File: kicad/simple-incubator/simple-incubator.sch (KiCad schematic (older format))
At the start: 17 parts, among them J1 Conn_Coaxial_Power, J2 Fan, J3 Onewire1, J4 FT232L, J5 Onewire2, Q1 BSP75, Q2 IRF3704, SW1 Rotary_Encoder_Switch, U1 MCP1703A-5002_SOT223, U2 ATmega328-AU

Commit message: update kicad
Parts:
- Q1: symbol BSP75:BSP75 -> simple-incubator-rescue:BSP75-BSP75
- R2: footprint (none) -> Resistor_SMD:R_0805_2012Metric_Pad1.15x1.40mm_HandSolder
- SP1: symbol ICSP:ICSP -> simple-incubator-rescue:ICSP-ICSP
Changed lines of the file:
@@
 $EndComp
 $Comp
-L BSP75:BSP75 Q1
+L simple-incubator-rescue:BSP75-BSP75 Q1
 U 1 1 5C8944AE
 P 6950 2900
@@
 $EndComp
 $Comp
-L ICSP:ICSP SP1
+L simple-incubator-rescue:ICSP-ICSP SP1
 U 1 1 5C8952B3
 P 2550 5100
@@
 	9050 2950 9200 2950
 $Comp
-L power:GND #PWR?
+L power:GND #PWR0114
 U 1 1 5C89B676
 P 9200 2950
-F 0 "#PWR?" H 9200 2700 50  0001 C CNN
+F 0 "#PWR0114" H 9200 2700 50  0001 C CNN
 F 1 "GND" H 9205 2777 50  0000 C CNN
 F 2 "" H 9200 2950 50  0001 C CNN
@@
 F 0 "R2" V 9143 2850 50  0000 C CNN
 F 1 "R" V 9234 2850 50  0000 C CNN
-F 2 "" V 9280 2850 50  0001 C CNN
+F 2 "Resistor_SMD:R_0805_2012Metric_Pad1.15x1.40mm_HandSolder" V 9280 2850 50  0001 C CNN
 F 3 "~" H 9350 2850 50  0001 C CNN
 	1    9350 2850
@@
 	9250 2200 8650 2200
 $Comp
-L power:VCC #PWR?
+L power:VCC #PWR0115
 U 1 1 5C89FAE2
 P 8650 1850
-F 0 "#PWR?" H 8650 1700 50  0001 C CNN
+F 0 "#PWR0115" H 8650 1700 50  0001 C CNN
 F 1 "VCC" H 8667 2023 50  0000 C CNN
 F 2 "" H 8650 1850 50  0001 C CNN
@@
 RESET
 $Comp
-L power:GND #PWR?
+L power:GND #PWR0116
 U 1 1 5C8ACF03
 P 3200 5250
-F 0 "#PWR?" H 3200 5000 50  0001 C CNN
+F 0 "#PWR0116" H 3200 5000 50  0001 C CNN
 F 1 "GND" H 3205 5077 50  0000 C CNN
 F 2 "" H 3200 5250 50  0001 C CNN
@@
 	3350 3550 3550 3550
 $Comp
-L power:GND #PWR?
+L power:GND #PWR0117
 U 1 1 5C8B7EBD
 P 3550 3350
-F 0 "#PWR?" H 3550 3100 50  0001 C CNN
+F 0 "#PWR0117" H 3550 3100 50  0001 C CNN
 F 1 "GND" H 3555 3177 50  0000 C CNN
 F 2 "" H 3550 3350 50  0001 C CNN
@@
 	2750 3450 2200 3450
 $Comp
-L power:GND #PWR?
+L power:GND #PWR0118
 U 1 1 5C8BA7E6
 P 2200 3450
-F 0 "#PWR?" H 2200 3200 50  0001 C CNN
+F 0 "#PWR0118" H 2200 3200 50  0001 C CNN
 F 1 "GND" H 2205 3277 50  0000 C CNN
 F 2 "" H 2200 3450 50  0001 C CNN

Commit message: The footprint should have changed to simple footprint design with 9 pads and a hole.
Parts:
- Q1: symbol simple-incubator-rescue:BSP75-BSP75 -> simple-incubator-rescue:BSP75-BSP75-simple-incubator-rescue
- SP1: symbol simple-incubator-rescue:ICSP-ICSP -> simple-incubator-rescue:ICSP-ICSP-simple-incubator-rescue
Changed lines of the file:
@@
 $EndComp
 $Comp
-L simple-incubator-rescue:BSP75-BSP75 Q1
+L simple-incubator-rescue:BSP75-BSP75-simple-incubator-rescue Q1
 U 1 1 5C8944AE
 P 6950 2900
@@
 $EndComp
 $Comp
-L simple-incubator-rescue:ICSP-ICSP SP1
+L simple-incubator-rescue:ICSP-ICSP-simple-incubator-rescue SP1
 U 1 1 5C8952B3
 P 2550 5100

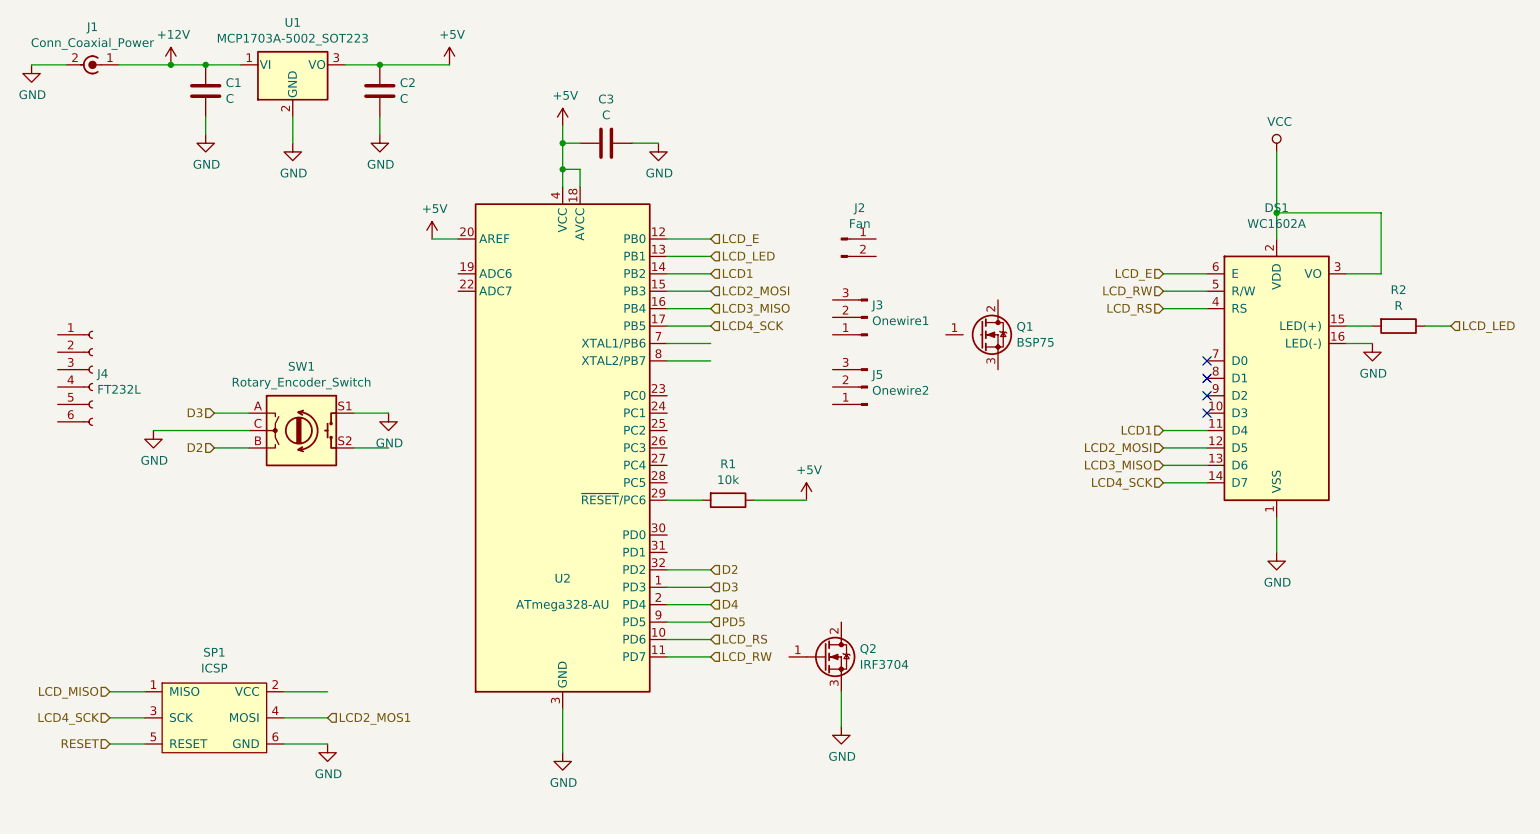
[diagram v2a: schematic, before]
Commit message: last weeks updates
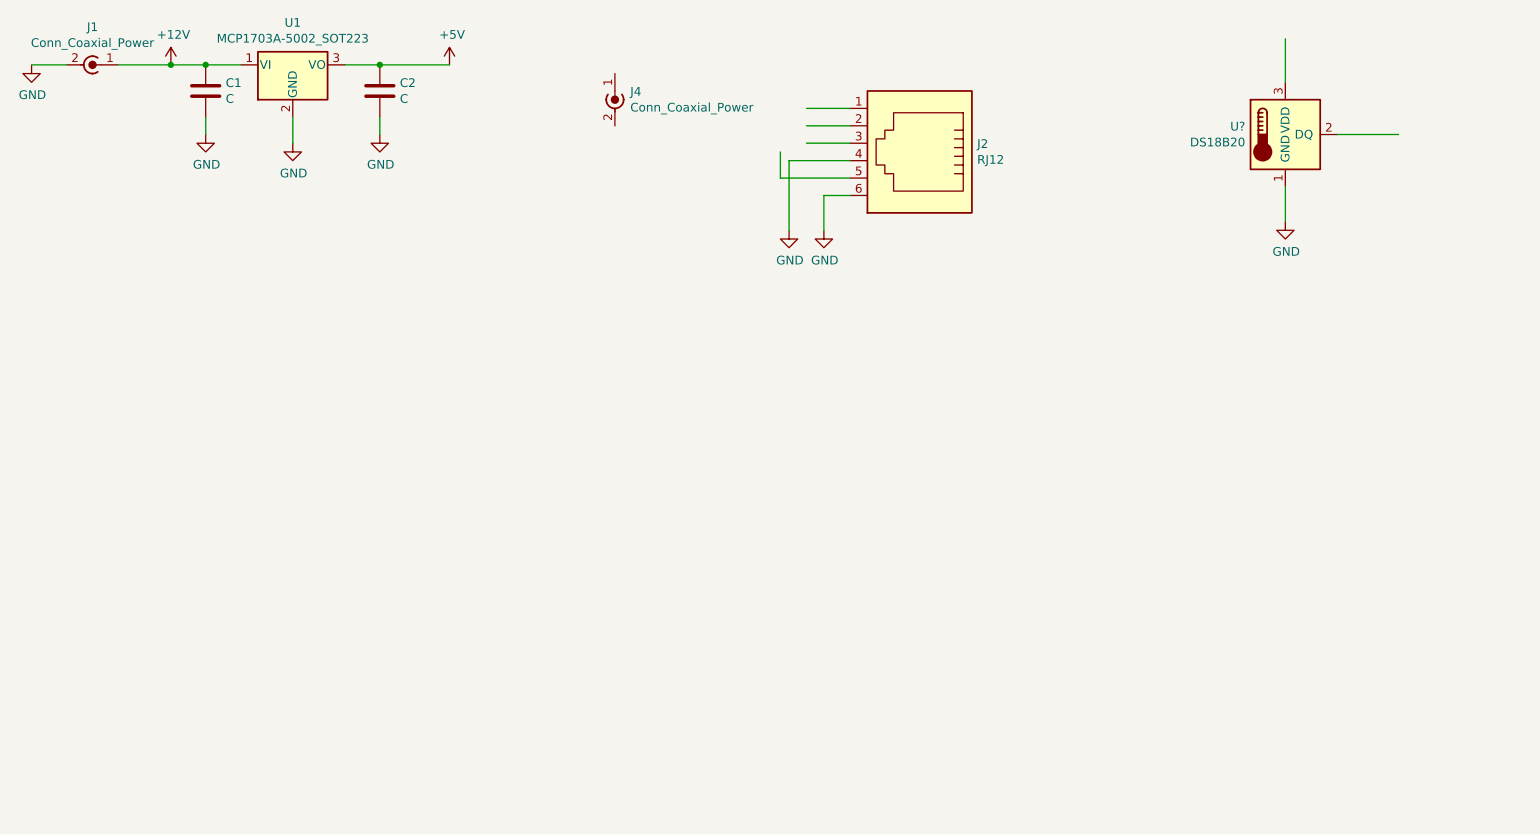
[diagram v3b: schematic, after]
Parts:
- removed C3: C, Capacitor_SMD:C_0805_2012Metric_Pad1.15x1.40mm_HandSolder, symbol Device:C
- removed DS1: WC1602A, Display:WC1602A, symbol Display_Character:WC1602A
- removed J2: Fan, Connector_BarrelJack:BarrelJack_Horizontal, symbol Connector:Conn_01x02_Male
- removed J3: Onewire1, Connector_Molex:Molex_KK-254_AE-6410-03A_1x03_P2.54mm_Vertical, symbol Connector:Conn_01x03_Male
- removed J4: FT232L, Connector_Molex:Molex_KK-254_AE-6410-06A_1x06_P2.54mm_Vertical, symbol Connector:Conn_01x06_Female
- removed J5: Onewire2, Connector_Molex:Molex_KK-254_AE-6410-04A_1x04_P2.54mm_Vertical, symbol Connector:Conn_01x03_Male
- removed Q1: BSP75, Package_TO_SOT_SMD:SOT-223-3_TabPin2, symbol simple-incubator-rescue:BSP75-BSP75-simple-incubator-rescue
- removed Q2: IRF3704, Package_TO_SOT_THT:TO-220-3_Vertical, symbol Transistor_FET:IRF3205
- removed R1: 10k, Resistor_SMD:R_0805_2012Metric_Pad1.15x1.40mm_HandSolder, symbol Device:R
- removed R2: R, Resistor_SMD:R_0805_2012Metric_Pad1.15x1.40mm_HandSolder, symbol Device:R
- removed SP1: ICSP, Connector:Tag-Connect_TC2030-IDC-NL_2x03_P1.27mm_Vertical, symbol simple-incubator-rescue:ICSP-ICSP-simple-incubator-rescue
- removed SW1: Rotary_Encoder_Switch, Rotary_Encoder:RotaryEncoder_Alps_EC11E-Switch_Vertical_H20mm, symbol Device:Rotary_Encoder_Switch
- removed U2: ATmega328-AU, Package_QFP:TQFP-32_7x7mm_P0.8mm, symbol MCU_Microchip_ATmega:ATmega328-AU
- added J2: RJ12, Connector_RJ:RJ12_Amphenol_54601, symbol Connector:RJ12
- added J4: Conn_Coaxial_Power, Connector_Coaxial:SMA_Amphenol_132134-11_Vertical, symbol Connector:Conn_Coaxial_Power
- added U?: DS18B20, Package_TO_SOT_THT:TO-92_Inline, symbol Sensor_Temperature:DS18B20
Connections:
- net labels removed: D2, D3, D4, LCD1, LCD2_MOS1, LCD2_MOSI, LCD3_MISO, LCD4_SCK, LCD_E, LCD_LED, LCD_MISO, LCD_RS, LCD_RW, PD5, RESET, VCC
- wire segments 62 -> 21
- no-connect marks 4 -> 0
